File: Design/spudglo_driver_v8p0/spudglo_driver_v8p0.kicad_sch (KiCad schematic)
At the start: 25 parts, among them J3 terminal_custom_12pin, U1 rf_433MHz_module, U12 USB-C-31-M-12, U13 XR21B1411, U14 NCP361, U2 rf_433MHz_module, U3 rf_433MHz_module, U4 rf_433MHz_module

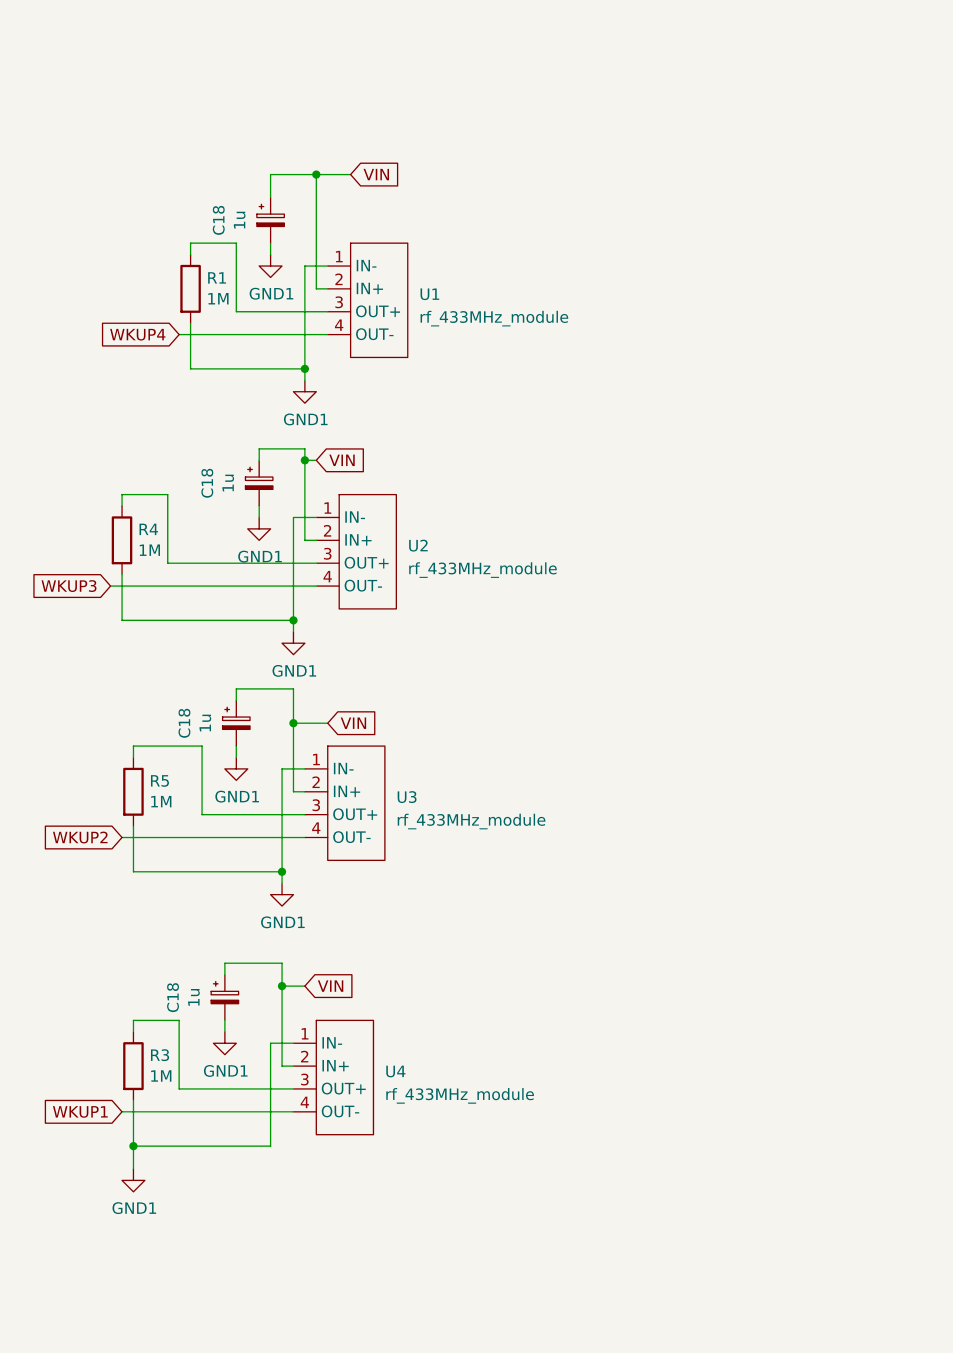
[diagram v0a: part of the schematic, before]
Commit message: add new spudglo boards
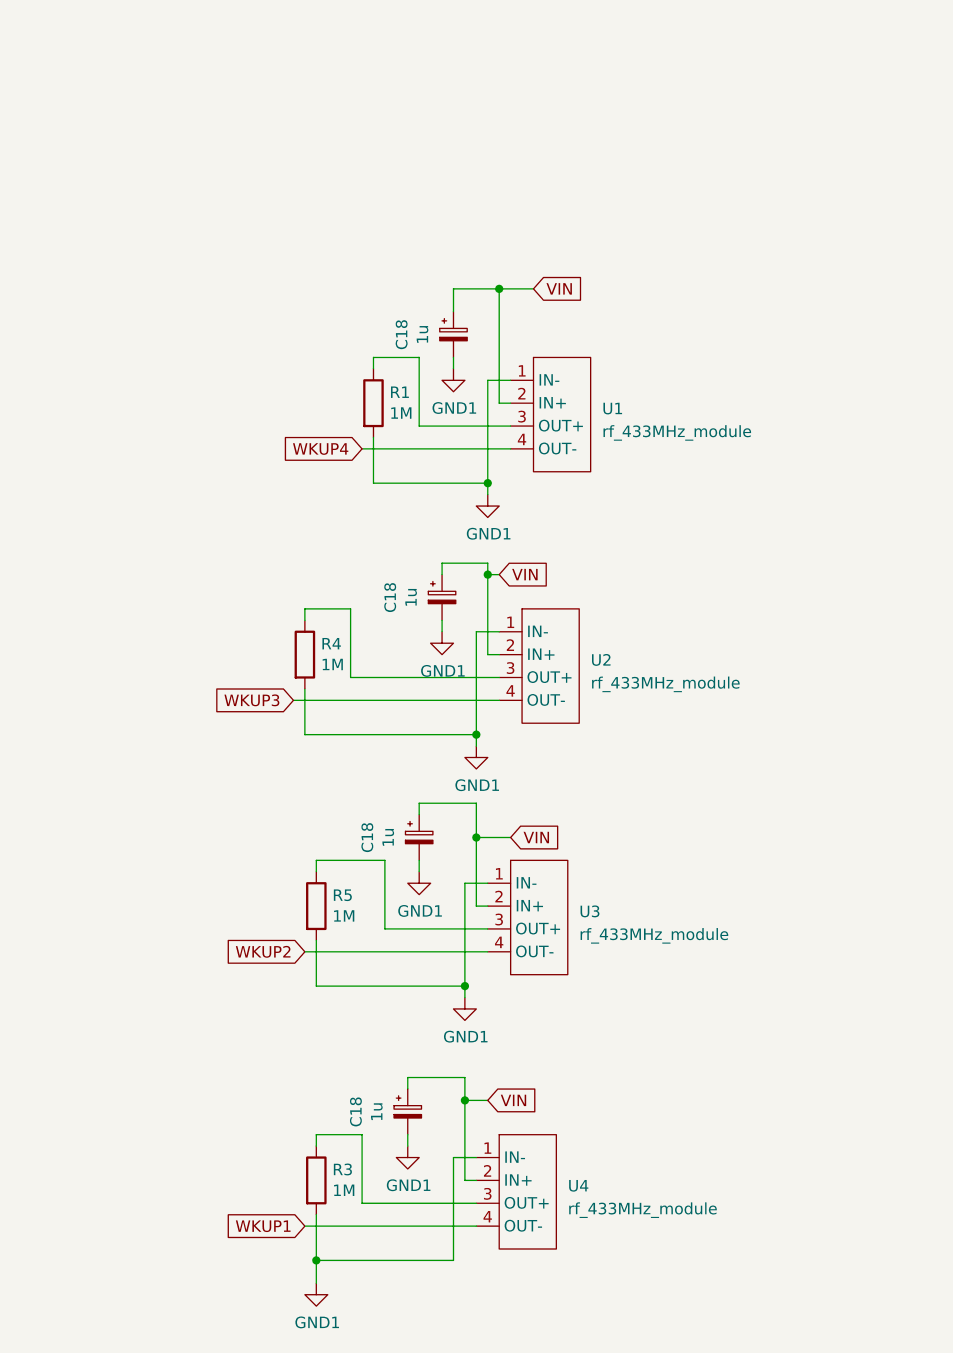
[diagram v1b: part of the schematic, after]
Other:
- moved on the sheet: C18, R1, R3, R4, R5, U1, U2, U3, U4
